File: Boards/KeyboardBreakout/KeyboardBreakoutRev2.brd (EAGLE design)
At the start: 86.8 x 21.8 mm, 2 parts

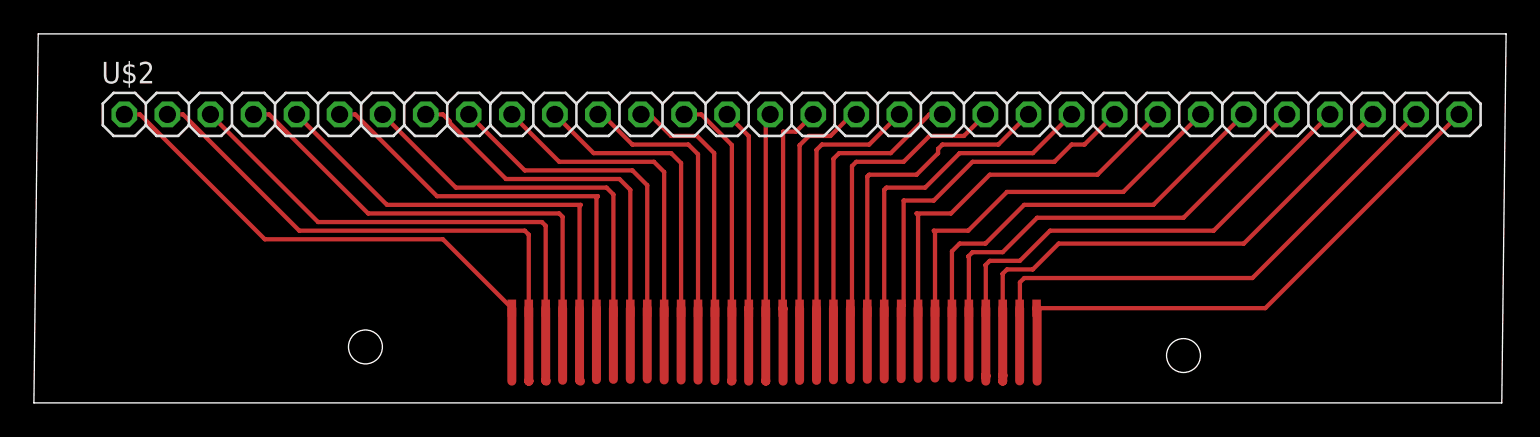
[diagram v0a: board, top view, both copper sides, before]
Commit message: Keyboard BreakoutRev2
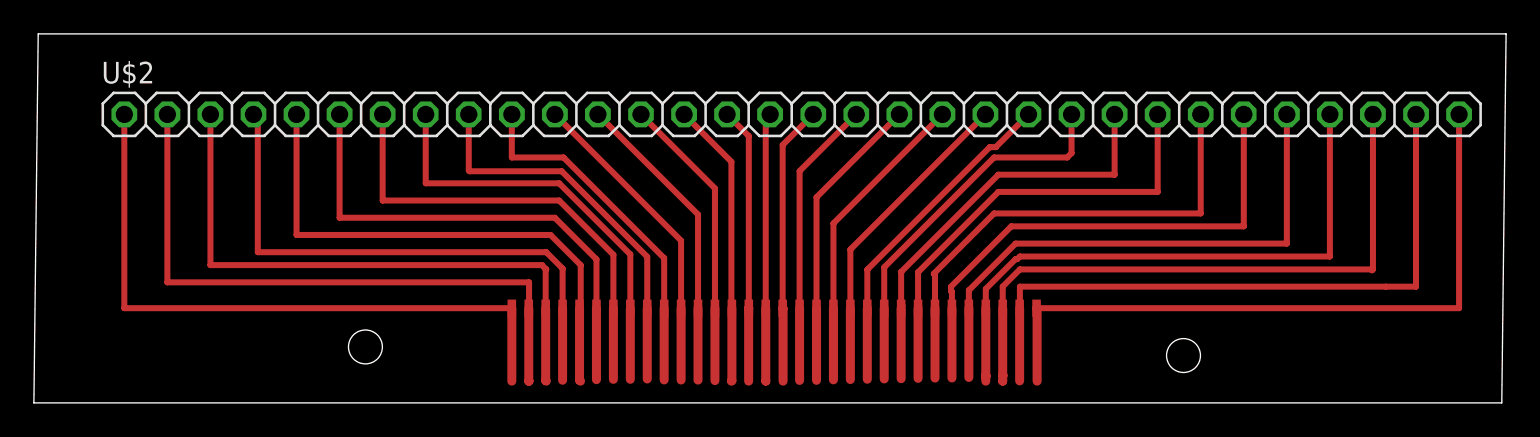
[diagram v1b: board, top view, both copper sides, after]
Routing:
- net N$32: track 31.9 -> 38.6 mm
- net N$1: track 34.0 -> 40.7 mm
- net N$2: track 33.3 -> 39.1 mm
- net N$3: track 32.1 -> 37.1 mm
- net N$31: track 32.9 -> 37.1 mm
- net N$4: track 31.0 -> 35.0 mm
- net N$30: track 31.7 -> 35.4 mm
- net N$11: track 23.1 -> 19.8 mm
- net N$5: track 29.4 -> 32.7 mm
- net N$28: track 29.4 -> 32.3 mm
- net N$29: track 30.4 -> 33.2 mm
- net N$6: track 28.0 -> 30.8 mm
- net N$12: track 21.8 -> 19.1 mm
- net N$22: track 21.4 -> 18.8 mm
- net N$13: track 20.6 -> 18.3 mm
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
